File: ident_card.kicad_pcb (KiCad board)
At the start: 2 copper layers, 49.5 x 29.8 mm, 47 parts, among them J1 Conn_02x10_Odd_Even, J2 Conn_02x07_Odd_Even, J3 USB_C_Receptacle_USB2.0, J4 Conn_01x02_Female, SW1 SW_Push, SW2 SW_SPDT, U1 STM32F303K8Tx, U2 CH340E, U3 MCP73831-2-OT, U4 ADP151_TSOT, Y1 32.768kHz

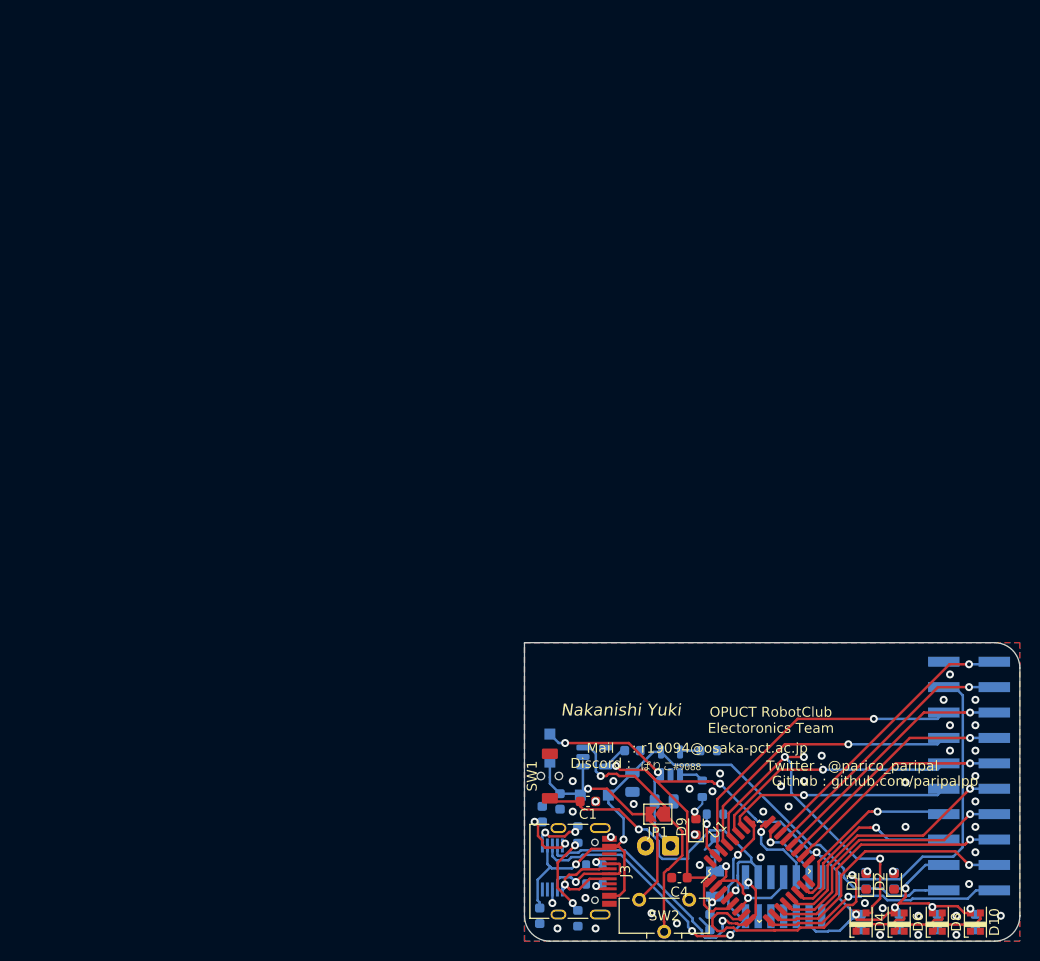
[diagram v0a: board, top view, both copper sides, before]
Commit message: arrayed
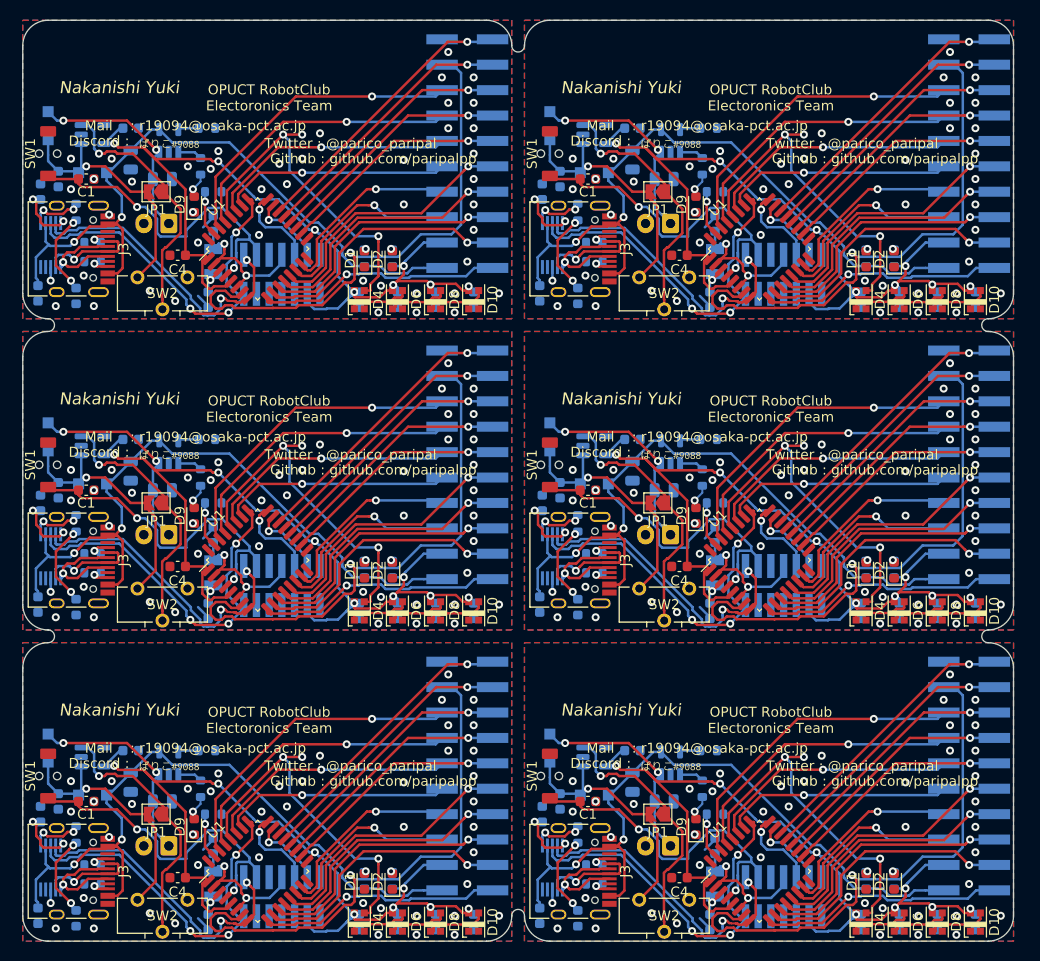
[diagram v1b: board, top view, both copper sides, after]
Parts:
- added C1: 0.1uF, Capacitor_SMD:C_0603_1608Metric, F.Cu at (84.5, 38.1)
- added C1: 0.1uF, Capacitor_SMD:C_0603_1608Metric, F.Cu at (84.5, 69.2)
- added C1: 0.1uF, Capacitor_SMD:C_0603_1608Metric, F.Cu at (84.5, 100.3)
- added C1: 0.1uF, Capacitor_SMD:C_0603_1608Metric, F.Cu at (134.6, 38.1)
- added C1: 0.1uF, Capacitor_SMD:C_0603_1608Metric, F.Cu at (134.6, 69.2)
- added C10: 0.1uF, Capacitor_SMD:C_0603_1608Metric, B.Cu at (115.6, 50.2)
- added C10: 0.1uF, Capacitor_SMD:C_0603_1608Metric, B.Cu at (115.6, 81.3)
- added C10: 0.1uF, Capacitor_SMD:C_0603_1608Metric, B.Cu at (115.6, 112.4)
- added C10: 0.1uF, Capacitor_SMD:C_0603_1608Metric, B.Cu at (165.7, 50.2)
- added C10: 0.1uF, Capacitor_SMD:C_0603_1608Metric, B.Cu at (165.7, 81.3)
- added C11: 0.1uF, Capacitor_SMD:C_0603_1608Metric, B.Cu at (119.4, 50.2)
- added C11: 0.1uF, Capacitor_SMD:C_0603_1608Metric, B.Cu at (119.4, 81.3)
- added C11: 0.1uF, Capacitor_SMD:C_0603_1608Metric, B.Cu at (119.4, 112.4)
- added C11: 0.1uF, Capacitor_SMD:C_0603_1608Metric, B.Cu at (169.5, 50.2)
- added C11: 0.1uF, Capacitor_SMD:C_0603_1608Metric, B.Cu at (169.5, 81.3)
- added C12: 0.1uF, Capacitor_SMD:C_0603_1608Metric, B.Cu at (123.2, 50.2)
- added C12: 0.1uF, Capacitor_SMD:C_0603_1608Metric, B.Cu at (123.2, 81.3)
- added C12: 0.1uF, Capacitor_SMD:C_0603_1608Metric, B.Cu at (123.2, 112.4)
- added C12: 0.1uF, Capacitor_SMD:C_0603_1608Metric, B.Cu at (173.4, 50.2)
- added C12: 0.1uF, Capacitor_SMD:C_0603_1608Metric, B.Cu at (173.4, 81.3)
- added C13: 10uF, Capacitor_SMD:C_0805_2012Metric, B.Cu at (92.1, 38.1)
- added C13: 10uF, Capacitor_SMD:C_0805_2012Metric, B.Cu at (92.1, 69.2)
- added C13: 10uF, Capacitor_SMD:C_0805_2012Metric, B.Cu at (92.1, 100.3)
- added C13: 10uF, Capacitor_SMD:C_0805_2012Metric, B.Cu at (142.2, 38.1)
- added C13: 10uF, Capacitor_SMD:C_0805_2012Metric, B.Cu at (142.2, 69.2)
- added C14: 1uF, Capacitor_SMD:C_0603_1608Metric, B.Cu at (88.9, 33.0)
- added C14: 1uF, Capacitor_SMD:C_0603_1608Metric, B.Cu at (88.9, 64.1)
- added C14: 1uF, Capacitor_SMD:C_0603_1608Metric, B.Cu at (88.9, 95.2)
- added C14: 1uF, Capacitor_SMD:C_0603_1608Metric, B.Cu at (139.1, 33.0)
- added C14: 1uF, Capacitor_SMD:C_0603_1608Metric, B.Cu at (139.1, 64.1)
- added C2: 15pF, Capacitor_SMD:C_0603_1608Metric, B.Cu at (97.2, 42.5)
- added C2: 15pF, Capacitor_SMD:C_0603_1608Metric, B.Cu at (97.2, 73.7)
- added C2: 15pF, Capacitor_SMD:C_0603_1608Metric, B.Cu at (97.2, 104.8)
- added C2: 15pF, Capacitor_SMD:C_0603_1608Metric, B.Cu at (147.3, 42.5)
- added C2: 15pF, Capacitor_SMD:C_0603_1608Metric, B.Cu at (147.3, 73.7)
- added C3: 15pF, Capacitor_SMD:C_0603_1608Metric, B.Cu at (96.6, 50.2)
- added C3: 15pF, Capacitor_SMD:C_0603_1608Metric, B.Cu at (96.6, 81.3)
- added C3: 15pF, Capacitor_SMD:C_0603_1608Metric, B.Cu at (96.6, 112.4)
- added C3: 15pF, Capacitor_SMD:C_0603_1608Metric, B.Cu at (146.8, 50.2)
- added C3: 15pF, Capacitor_SMD:C_0603_1608Metric, B.Cu at (146.8, 81.3)
- added C4: 0.1uF, Capacitor_SMD:C_0603_1608Metric, F.Cu at (93.6, 45.7)
- added C4: 0.1uF, Capacitor_SMD:C_0603_1608Metric, F.Cu at (93.6, 76.8)
- added C4: 0.1uF, Capacitor_SMD:C_0603_1608Metric, F.Cu at (93.6, 108.0)
- added C4: 0.1uF, Capacitor_SMD:C_0603_1608Metric, F.Cu at (143.8, 45.7)
- added C4: 0.1uF, Capacitor_SMD:C_0603_1608Metric, F.Cu at (143.8, 76.8)
- added C5: 0.1uF, Capacitor_SMD:C_0603_1608Metric, B.Cu at (79.9, 39.4)
- added C5: 0.1uF, Capacitor_SMD:C_0603_1608Metric, B.Cu at (79.9, 70.5)
- added C5: 0.1uF, Capacitor_SMD:C_0603_1608Metric, B.Cu at (79.9, 101.6)
- added C5: 0.1uF, Capacitor_SMD:C_0603_1608Metric, B.Cu at (130.0, 39.4)
- added C5: 0.1uF, Capacitor_SMD:C_0603_1608Metric, B.Cu at (130.0, 70.5)
- added C6: 0.1uF, Capacitor_SMD:C_0603_1608Metric, B.Cu at (79.6, 49.5)
- added C6: 0.1uF, Capacitor_SMD:C_0603_1608Metric, B.Cu at (79.6, 80.6)
- added C6: 0.1uF, Capacitor_SMD:C_0603_1608Metric, B.Cu at (79.6, 111.8)
- added C6: 0.1uF, Capacitor_SMD:C_0603_1608Metric, B.Cu at (129.8, 49.5)
- added C6: 0.1uF, Capacitor_SMD:C_0603_1608Metric, B.Cu at (129.8, 80.6)
- added C7: 10uF, Capacitor_SMD:C_0805_2012Metric, B.Cu at (88.9, 36.2)
- added C7: 10uF, Capacitor_SMD:C_0805_2012Metric, B.Cu at (88.9, 67.3)
- added C7: 10uF, Capacitor_SMD:C_0805_2012Metric, B.Cu at (88.9, 98.4)
- added C7: 10uF, Capacitor_SMD:C_0805_2012Metric, B.Cu at (139.1, 36.2)
- added C7: 10uF, Capacitor_SMD:C_0805_2012Metric, B.Cu at (139.1, 67.3)
- added C8: 0.1uF, Capacitor_SMD:C_0603_1608Metric, B.Cu at (111.8, 50.2)
- added C8: 0.1uF, Capacitor_SMD:C_0603_1608Metric, B.Cu at (111.8, 81.3)
- added C8: 0.1uF, Capacitor_SMD:C_0603_1608Metric, B.Cu at (111.8, 112.4)
- added C8: 0.1uF, Capacitor_SMD:C_0603_1608Metric, B.Cu at (161.9, 50.2)
- added C8: 0.1uF, Capacitor_SMD:C_0603_1608Metric, B.Cu at (161.9, 81.3)
- added C9: 1uF, Capacitor_SMD:C_0603_1608Metric, B.Cu at (81.7, 38.1)
- added C9: 1uF, Capacitor_SMD:C_0603_1608Metric, B.Cu at (81.7, 69.2)
- added C9: 1uF, Capacitor_SMD:C_0603_1608Metric, B.Cu at (81.7, 100.3)
- added C9: 1uF, Capacitor_SMD:C_0603_1608Metric, B.Cu at (131.8, 38.1)
- added C9: 1uF, Capacitor_SMD:C_0603_1608Metric, B.Cu at (131.8, 69.2)
- added D1: LED, LED_SMD:LED_0603_1608Metric, F.Cu at (112.3, 46.1)
- added D1: LED, LED_SMD:LED_0603_1608Metric, F.Cu at (112.3, 77.2)
- added D1: LED, LED_SMD:LED_0603_1608Metric, F.Cu at (112.3, 108.3)
- added D1: LED, LED_SMD:LED_0603_1608Metric, F.Cu at (162.4, 46.1)
- added D1: LED, LED_SMD:LED_0603_1608Metric, F.Cu at (162.4, 77.2)
- added D10: WS2812C, LED_additional:LED_2020Metric_WS2812C_2.0x2.0mm_P1.0mm, F.Cu at (123.2, 50.2)
- added D10: WS2812C, LED_additional:LED_2020Metric_WS2812C_2.0x2.0mm_P1.0mm, F.Cu at (123.2, 81.3)
- added D10: WS2812C, LED_additional:LED_2020Metric_WS2812C_2.0x2.0mm_P1.0mm, F.Cu at (123.2, 112.4)
- added D10: WS2812C, LED_additional:LED_2020Metric_WS2812C_2.0x2.0mm_P1.0mm, F.Cu at (173.4, 50.2)
- added D10: WS2812C, LED_additional:LED_2020Metric_WS2812C_2.0x2.0mm_P1.0mm, F.Cu at (173.4, 81.3)
- added D2: LED, LED_SMD:LED_0603_1608Metric, F.Cu at (115.1, 46.1)
- added D2: LED, LED_SMD:LED_0603_1608Metric, F.Cu at (115.1, 77.2)
- added D2: LED, LED_SMD:LED_0603_1608Metric, F.Cu at (115.1, 108.3)
- added D2: LED, LED_SMD:LED_0603_1608Metric, F.Cu at (165.2, 46.1)
- added D2: LED, LED_SMD:LED_0603_1608Metric, F.Cu at (165.2, 77.2)
- added D3: LED, LED_SMD:LED_0603_1608Metric, B.Cu at (83.4, 49.8)
- added D3: LED, LED_SMD:LED_0603_1608Metric, B.Cu at (83.4, 80.9)
- added D3: LED, LED_SMD:LED_0603_1608Metric, B.Cu at (83.4, 112.0)
- added D3: LED, LED_SMD:LED_0603_1608Metric, B.Cu at (133.6, 49.8)
- added D3: LED, LED_SMD:LED_0603_1608Metric, B.Cu at (133.6, 80.9)
- added D4: WS2812C, LED_additional:LED_2020Metric_WS2812C_2.0x2.0mm_P1.0mm, F.Cu at (111.8, 50.2)
- added D4: WS2812C, LED_additional:LED_2020Metric_WS2812C_2.0x2.0mm_P1.0mm, F.Cu at (111.8, 81.3)
- added D4: WS2812C, LED_additional:LED_2020Metric_WS2812C_2.0x2.0mm_P1.0mm, F.Cu at (111.8, 112.4)
- added D4: WS2812C, LED_additional:LED_2020Metric_WS2812C_2.0x2.0mm_P1.0mm, F.Cu at (161.9, 50.2)
- added D4: WS2812C, LED_additional:LED_2020Metric_WS2812C_2.0x2.0mm_P1.0mm, F.Cu at (161.9, 81.3)
- added D5: D, Diode_SMD:D_SOD-123F, B.Cu at (80.6, 32.8)
- added D5: D, Diode_SMD:D_SOD-123F, B.Cu at (80.6, 63.9)
- added D5: D, Diode_SMD:D_SOD-123F, B.Cu at (80.6, 95.0)
- added D5: D, Diode_SMD:D_SOD-123F, B.Cu at (130.8, 32.8)
- added D5: D, Diode_SMD:D_SOD-123F, B.Cu at (130.8, 63.9)
- added D6: WS2812C, LED_additional:LED_2020Metric_WS2812C_2.0x2.0mm_P1.0mm, F.Cu at (115.6, 50.2)
- added D6: WS2812C, LED_additional:LED_2020Metric_WS2812C_2.0x2.0mm_P1.0mm, F.Cu at (115.6, 81.3)
- added D6: WS2812C, LED_additional:LED_2020Metric_WS2812C_2.0x2.0mm_P1.0mm, F.Cu at (115.6, 112.4)
- added D6: WS2812C, LED_additional:LED_2020Metric_WS2812C_2.0x2.0mm_P1.0mm, F.Cu at (165.7, 50.2)
- added D6: WS2812C, LED_additional:LED_2020Metric_WS2812C_2.0x2.0mm_P1.0mm, F.Cu at (165.7, 81.3)
- added D7: D, Diode_SMD:D_SOD-123F, B.Cu at (85.1, 37.5)
- added D7: D, Diode_SMD:D_SOD-123F, B.Cu at (85.1, 68.6)
- added D7: D, Diode_SMD:D_SOD-123F, B.Cu at (85.1, 99.7)
- added D7: D, Diode_SMD:D_SOD-123F, B.Cu at (135.3, 37.5)
- added D7: D, Diode_SMD:D_SOD-123F, B.Cu at (135.3, 68.6)
- added D8: WS2812C, LED_additional:LED_2020Metric_WS2812C_2.0x2.0mm_P1.0mm, F.Cu at (119.4, 50.2)
- added D8: WS2812C, LED_additional:LED_2020Metric_WS2812C_2.0x2.0mm_P1.0mm, F.Cu at (119.4, 81.3)
- added D8: WS2812C, LED_additional:LED_2020Metric_WS2812C_2.0x2.0mm_P1.0mm, F.Cu at (119.4, 112.4)
- added D8: WS2812C, LED_additional:LED_2020Metric_WS2812C_2.0x2.0mm_P1.0mm, F.Cu at (169.5, 50.2)
- added D8: WS2812C, LED_additional:LED_2020Metric_WS2812C_2.0x2.0mm_P1.0mm, F.Cu at (169.5, 81.3)
- added D9: LED, LED_SMD:LED_0603_1608Metric, F.Cu at (95.2, 40.6)
- added D9: LED, LED_SMD:LED_0603_1608Metric, F.Cu at (95.2, 71.8)
- added D9: LED, LED_SMD:LED_0603_1608Metric, F.Cu at (95.2, 102.9)
- added D9: LED, LED_SMD:LED_0603_1608Metric, F.Cu at (145.4, 40.6)
- added D9: LED, LED_SMD:LED_0603_1608Metric, F.Cu at (145.4, 71.8)
- added G***: LOGO, kicad_local_lib:twitter_qr_with_logo_19x19, B.Cu at (108.6, 34.5)
- added G***: LOGO, kicad_local_lib:twitter_qr_with_logo_19x19, B.Cu at (158.8, 34.5)
- added G***: LOGO, kicad_local_lib:github_qr_with_logo_9x9, B.Cu at (136.4, 27.4)
- added G***: LOGO, kicad_local_lib:discordname_8x3mm, F.Cu at (143.3, 34.8)
- added G***: LOGO, kicad_local_lib:twitter_qr_with_logo_19x19, B.Cu at (158.8, 65.7)
- added G***: LOGO, kicad_local_lib:github_qr_with_logo_9x9, B.Cu at (136.4, 58.5)
- added G***: LOGO, kicad_local_lib:discordname_8x3mm, F.Cu at (143.3, 65.9)
- added G***: LOGO, kicad_local_lib:github_qr_with_logo_9x9, B.Cu at (86.2, 27.4)
- added G***: LOGO, kicad_local_lib:discordname_8x3mm, F.Cu at (93.1, 34.8)
- added G***: LOGO, kicad_local_lib:twitter_qr_with_logo_19x19, B.Cu at (108.6, 65.7)
- added G***: LOGO, kicad_local_lib:github_qr_with_logo_9x9, B.Cu at (86.2, 58.5)
- added G***: LOGO, kicad_local_lib:discordname_8x3mm, F.Cu at (93.1, 65.9)
- added G***: LOGO, kicad_local_lib:twitter_qr_with_logo_19x19, B.Cu at (108.6, 96.8)
- added G***: LOGO, kicad_local_lib:github_qr_with_logo_9x9, B.Cu at (86.2, 89.7)
- added G***: LOGO, kicad_local_lib:discordname_8x3mm, F.Cu at (93.1, 97.0)
- added J1: Conn_02x10_Odd_Even, Connector_PinHeader_2.54mm:PinHeader_2x10_P2.54mm_Vertical_SMD, B.Cu at (122.6, 35.6)
- added J1: Conn_02x10_Odd_Even, Connector_PinHeader_2.54mm:PinHeader_2x10_P2.54mm_Vertical_SMD, B.Cu at (122.6, 66.7)
- added J1: Conn_02x10_Odd_Even, Connector_PinHeader_2.54mm:PinHeader_2x10_P2.54mm_Vertical_SMD, B.Cu at (122.6, 97.8)
- added J1: Conn_02x10_Odd_Even, Connector_PinHeader_2.54mm:PinHeader_2x10_P2.54mm_Vertical_SMD, B.Cu at (172.7, 35.6)
- added J1: Conn_02x10_Odd_Even, Connector_PinHeader_2.54mm:PinHeader_2x10_P2.54mm_Vertical_SMD, B.Cu at (172.7, 66.7)
- added J2: Conn_02x07_Odd_Even, Connector_PinHeader_1.27mm:PinHeader_2x07_P1.27mm_Vertical_SMD, B.Cu at (104.0, 47.6)
- added J2: Conn_02x07_Odd_Even, Connector_PinHeader_1.27mm:PinHeader_2x07_P1.27mm_Vertical_SMD, B.Cu at (104.0, 78.7)
- added J2: Conn_02x07_Odd_Even, Connector_PinHeader_1.27mm:PinHeader_2x07_P1.27mm_Vertical_SMD, B.Cu at (104.0, 109.9)
- added J2: Conn_02x07_Odd_Even, Connector_PinHeader_1.27mm:PinHeader_2x07_P1.27mm_Vertical_SMD, B.Cu at (154.2, 47.6)
- added J2: Conn_02x07_Odd_Even, Connector_PinHeader_1.27mm:PinHeader_2x07_P1.27mm_Vertical_SMD, B.Cu at (154.2, 78.7)
- added J3: USB_C_Receptacle_USB2.0, Connector_USB:USB_C_Receptacle_HRO_TYPE-C-31-M-12, F.Cu at (82.5, 45.1)
- added J3: USB_C_Receptacle_USB2.0, Connector_USB:USB_C_Receptacle_HRO_TYPE-C-31-M-12, F.Cu at (82.5, 76.2)
- added J3: USB_C_Receptacle_USB2.0, Connector_USB:USB_C_Receptacle_HRO_TYPE-C-31-M-12, F.Cu at (82.5, 107.3)
- added J3: USB_C_Receptacle_USB2.0, Connector_USB:USB_C_Receptacle_HRO_TYPE-C-31-M-12, F.Cu at (132.7, 45.1)
- added J3: USB_C_Receptacle_USB2.0, Connector_USB:USB_C_Receptacle_HRO_TYPE-C-31-M-12, F.Cu at (132.7, 76.2)
- added J4: Conn_01x02_Female, Connector_JST:JST_XA_S02B-XASK-1N-BN_1x02_P2.50mm_Horizontal, B.Cu at (92.7, 42.5)
- added J4: Conn_01x02_Female, Connector_JST:JST_XA_S02B-XASK-1N-BN_1x02_P2.50mm_Horizontal, B.Cu at (92.7, 73.7)
- added J4: Conn_01x02_Female, Connector_JST:JST_XA_S02B-XASK-1N-BN_1x02_P2.50mm_Horizontal, B.Cu at (92.7, 104.8)
- added J4: Conn_01x02_Female, Connector_JST:JST_XA_S02B-XASK-1N-BN_1x02_P2.50mm_Horizontal, B.Cu at (142.9, 42.5)
- added J4: Conn_01x02_Female, Connector_JST:JST_XA_S02B-XASK-1N-BN_1x02_P2.50mm_Horizontal, B.Cu at (142.9, 73.7)
- added JP1: SolderJumper_2_Open, Jumper:SolderJumper-2_P1.3mm_Open_TrianglePad1.0x1.5mm, F.Cu at (91.4, 39.4)
- added JP1: SolderJumper_2_Open, Jumper:SolderJumper-2_P1.3mm_Open_TrianglePad1.0x1.5mm, F.Cu at (91.4, 70.5)
- added JP1: SolderJumper_2_Open, Jumper:SolderJumper-2_P1.3mm_Open_TrianglePad1.0x1.5mm, F.Cu at (91.4, 101.6)
- added JP1: SolderJumper_2_Open, Jumper:SolderJumper-2_P1.3mm_Open_TrianglePad1.0x1.5mm, F.Cu at (141.6, 39.4)
- added JP1: SolderJumper_2_Open, Jumper:SolderJumper-2_P1.3mm_Open_TrianglePad1.0x1.5mm, F.Cu at (141.6, 70.5)
- added R1: 4.7kOhm, Resistor_SMD:R_0603_1608Metric, B.Cu at (112.3, 46.0)
- added R1: 4.7kOhm, Resistor_SMD:R_0603_1608Metric, B.Cu at (112.3, 77.1)
- added R1: 4.7kOhm, Resistor_SMD:R_0603_1608Metric, B.Cu at (112.3, 108.2)
- added R1: 4.7kOhm, Resistor_SMD:R_0603_1608Metric, B.Cu at (162.4, 46.0)
- added R1: 4.7kOhm, Resistor_SMD:R_0603_1608Metric, B.Cu at (162.4, 77.1)
- added R2: 4.7kOhm, Resistor_SMD:R_0603_1608Metric, B.Cu at (115.1, 46.0)
- added R2: 4.7kOhm, Resistor_SMD:R_0603_1608Metric, B.Cu at (115.1, 77.1)
- added R2: 4.7kOhm, Resistor_SMD:R_0603_1608Metric, B.Cu at (115.1, 108.2)
- added R2: 4.7kOhm, Resistor_SMD:R_0603_1608Metric, B.Cu at (165.2, 46.0)
- added R2: 4.7kOhm, Resistor_SMD:R_0603_1608Metric, B.Cu at (165.2, 77.1)
- added R3: 10kOhm, Resistor_SMD:R_0603_1608Metric, B.Cu at (97.2, 39.4)
- added R3: 10kOhm, Resistor_SMD:R_0603_1608Metric, B.Cu at (97.2, 70.5)
- added R3: 10kOhm, Resistor_SMD:R_0603_1608Metric, B.Cu at (97.2, 101.6)
- added R3: 10kOhm, Resistor_SMD:R_0603_1608Metric, B.Cu at (147.3, 39.4)
- added R3: 10kOhm, Resistor_SMD:R_0603_1608Metric, B.Cu at (147.3, 70.5)
- added R4: 5.1kOhm, Resistor_SMD:R_0603_1608Metric, B.Cu at (85.1, 44.5)
- added R4: 5.1kOhm, Resistor_SMD:R_0603_1608Metric, B.Cu at (85.1, 75.6)
- added R4: 5.1kOhm, Resistor_SMD:R_0603_1608Metric, B.Cu at (85.1, 106.7)
- added R4: 5.1kOhm, Resistor_SMD:R_0603_1608Metric, B.Cu at (135.3, 44.5)
- added R4: 5.1kOhm, Resistor_SMD:R_0603_1608Metric, B.Cu at (135.3, 75.6)
- added R5: 5.1kOhm, Resistor_SMD:R_0603_1608Metric, B.Cu at (85.1, 46.4)
- added R5: 5.1kOhm, Resistor_SMD:R_0603_1608Metric, B.Cu at (85.1, 77.5)
- added R5: 5.1kOhm, Resistor_SMD:R_0603_1608Metric, B.Cu at (85.1, 108.6)
- added R5: 5.1kOhm, Resistor_SMD:R_0603_1608Metric, B.Cu at (135.3, 46.4)
- added R5: 5.1kOhm, Resistor_SMD:R_0603_1608Metric, B.Cu at (135.3, 77.5)
- added R6: 470Ohm, Resistor_SMD:R_0603_1608Metric, B.Cu at (83.4, 41.4)
- added R6: 470Ohm, Resistor_SMD:R_0603_1608Metric, B.Cu at (83.4, 72.5)
- added R6: 470Ohm, Resistor_SMD:R_0603_1608Metric, B.Cu at (83.4, 103.6)
- added R6: 470Ohm, Resistor_SMD:R_0603_1608Metric, B.Cu at (133.6, 41.4)
- added R6: 470Ohm, Resistor_SMD:R_0603_1608Metric, B.Cu at (133.6, 72.5)
- added R7: 10kOhm, Resistor_SMD:R_0603_1608Metric, B.Cu at (96.5, 33.0)
- added R7: 10kOhm, Resistor_SMD:R_0603_1608Metric, B.Cu at (96.5, 64.1)
- added R7: 10kOhm, Resistor_SMD:R_0603_1608Metric, B.Cu at (96.5, 95.2)
- added R7: 10kOhm, Resistor_SMD:R_0603_1608Metric, B.Cu at (146.7, 33.0)
- added R7: 10kOhm, Resistor_SMD:R_0603_1608Metric, B.Cu at (146.7, 64.1)
- added R8: 470Ohm, Resistor_SMD:R_0603_1608Metric, B.Cu at (95.9, 36.8)
- added R8: 470Ohm, Resistor_SMD:R_0603_1608Metric, B.Cu at (95.9, 67.9)
- added R8: 470Ohm, Resistor_SMD:R_0603_1608Metric, B.Cu at (95.9, 99.1)
- added R8: 470Ohm, Resistor_SMD:R_0603_1608Metric, B.Cu at (146.1, 36.8)
- added R8: 470Ohm, Resistor_SMD:R_0603_1608Metric, B.Cu at (146.1, 67.9)
- added SW1: SW_Push, Button_Switch_additional:TVAF06-A020B-R, F.Cu at (80.6, 35.6)
- added SW1: SW_Push, Button_Switch_additional:TVAF06-A020B-R, F.Cu at (80.6, 66.7)
- added SW1: SW_Push, Button_Switch_additional:TVAF06-A020B-R, F.Cu at (80.6, 97.8)
- added SW1: SW_Push, Button_Switch_additional:TVAF06-A020B-R, F.Cu at (130.8, 35.6)
- added SW1: SW_Push, Button_Switch_additional:TVAF06-A020B-R, F.Cu at (130.8, 66.7)
- added SW2: SW_SPDT, Button_Switch_additional:IS-1245T-G, F.Cu at (92.1, 49.5)
- added SW2: SW_SPDT, Button_Switch_additional:IS-1245T-G, F.Cu at (92.1, 80.6)
- added SW2: SW_SPDT, Button_Switch_additional:IS-1245T-G, F.Cu at (92.1, 111.8)
- added SW2: SW_SPDT, Button_Switch_additional:IS-1245T-G, F.Cu at (142.2, 49.5)
- added SW2: SW_SPDT, Button_Switch_additional:IS-1245T-G, F.Cu at (142.2, 80.6)
- added U1: STM32F303K8Tx, Package_QFP:LQFP-32_7x7mm_P0.8mm, F.Cu at (101.6, 45.1)
- added U1: STM32F303K8Tx, Package_QFP:LQFP-32_7x7mm_P0.8mm, F.Cu at (101.6, 76.2)
- added U1: STM32F303K8Tx, Package_QFP:LQFP-32_7x7mm_P0.8mm, F.Cu at (101.6, 107.3)
- added U1: STM32F303K8Tx, Package_QFP:LQFP-32_7x7mm_P0.8mm, F.Cu at (151.8, 45.1)
- added U1: STM32F303K8Tx, Package_QFP:LQFP-32_7x7mm_P0.8mm, F.Cu at (151.8, 76.2)
- added U2: CH340E, Package_SO:MSOP-10_3x3mm_P0.5mm, B.Cu at (80.9, 44.7)
- added U2: CH340E, Package_SO:MSOP-10_3x3mm_P0.5mm, B.Cu at (80.9, 75.8)
- added U2: CH340E, Package_SO:MSOP-10_3x3mm_P0.5mm, B.Cu at (80.9, 106.9)
- added U2: CH340E, Package_SO:MSOP-10_3x3mm_P0.5mm, B.Cu at (131.1, 44.7)
- added U2: CH340E, Package_SO:MSOP-10_3x3mm_P0.5mm, B.Cu at (131.1, 75.8)
- added U3: MCP73831-2-OT, Package_TO_SOT_SMD:SOT-23-5, B.Cu at (92.7, 34.3)
- added U3: MCP73831-2-OT, Package_TO_SOT_SMD:SOT-23-5, B.Cu at (92.7, 65.4)
- added U3: MCP73831-2-OT, Package_TO_SOT_SMD:SOT-23-5, B.Cu at (92.7, 96.5)
- added U3: MCP73831-2-OT, Package_TO_SOT_SMD:SOT-23-5, B.Cu at (142.9, 34.3)
- added U3: MCP73831-2-OT, Package_TO_SOT_SMD:SOT-23-5, B.Cu at (142.9, 65.4)
- added U4: ADP151_TSOT, Package_TO_SOT_SMD:TSOT-23-5, B.Cu at (85.1, 33.7)
- added U4: ADP151_TSOT, Package_TO_SOT_SMD:TSOT-23-5, B.Cu at (85.1, 64.8)
- added U4: ADP151_TSOT, Package_TO_SOT_SMD:TSOT-23-5, B.Cu at (85.1, 95.9)
- added U4: ADP151_TSOT, Package_TO_SOT_SMD:TSOT-23-5, B.Cu at (135.3, 33.7)
- added U4: ADP151_TSOT, Package_TO_SOT_SMD:TSOT-23-5, B.Cu at (135.3, 64.8)
- added Y1: 32.768kHz, Crystal_additional:Crystal_SMD_SeikoEpson_FC135-2Pin_3.2x1.5mm, B.Cu at (97.2, 46.4)
- added Y1: 32.768kHz, Crystal_additional:Crystal_SMD_SeikoEpson_FC135-2Pin_3.2x1.5mm, B.Cu at (97.2, 77.5)
- added Y1: 32.768kHz, Crystal_additional:Crystal_SMD_SeikoEpson_FC135-2Pin_3.2x1.5mm, B.Cu at (97.2, 108.6)
- added Y1: 32.768kHz, Crystal_additional:Crystal_SMD_SeikoEpson_FC135-2Pin_3.2x1.5mm, B.Cu at (147.3, 46.4)
- added Y1: 32.768kHz, Crystal_additional:Crystal_SMD_SeikoEpson_FC135-2Pin_3.2x1.5mm, B.Cu at (147.3, 77.5)
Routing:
- net (no net): track 0.00 -> 4757.7 mm, vias 0 -> 525
- added copper zone on B.Cu, net (none)
- added copper zone on F.Cu, net (none)
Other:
- board size 49.5 x 29.8 mm -> 99.1 x 92.1 mm
